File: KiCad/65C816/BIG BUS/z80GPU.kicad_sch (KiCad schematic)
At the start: 12 parts, among them J8 Bus Header, U12 74LS573, U13 74LS573, U14 74LS573, U15 74HC00, U16 CTC, U17 74HC02

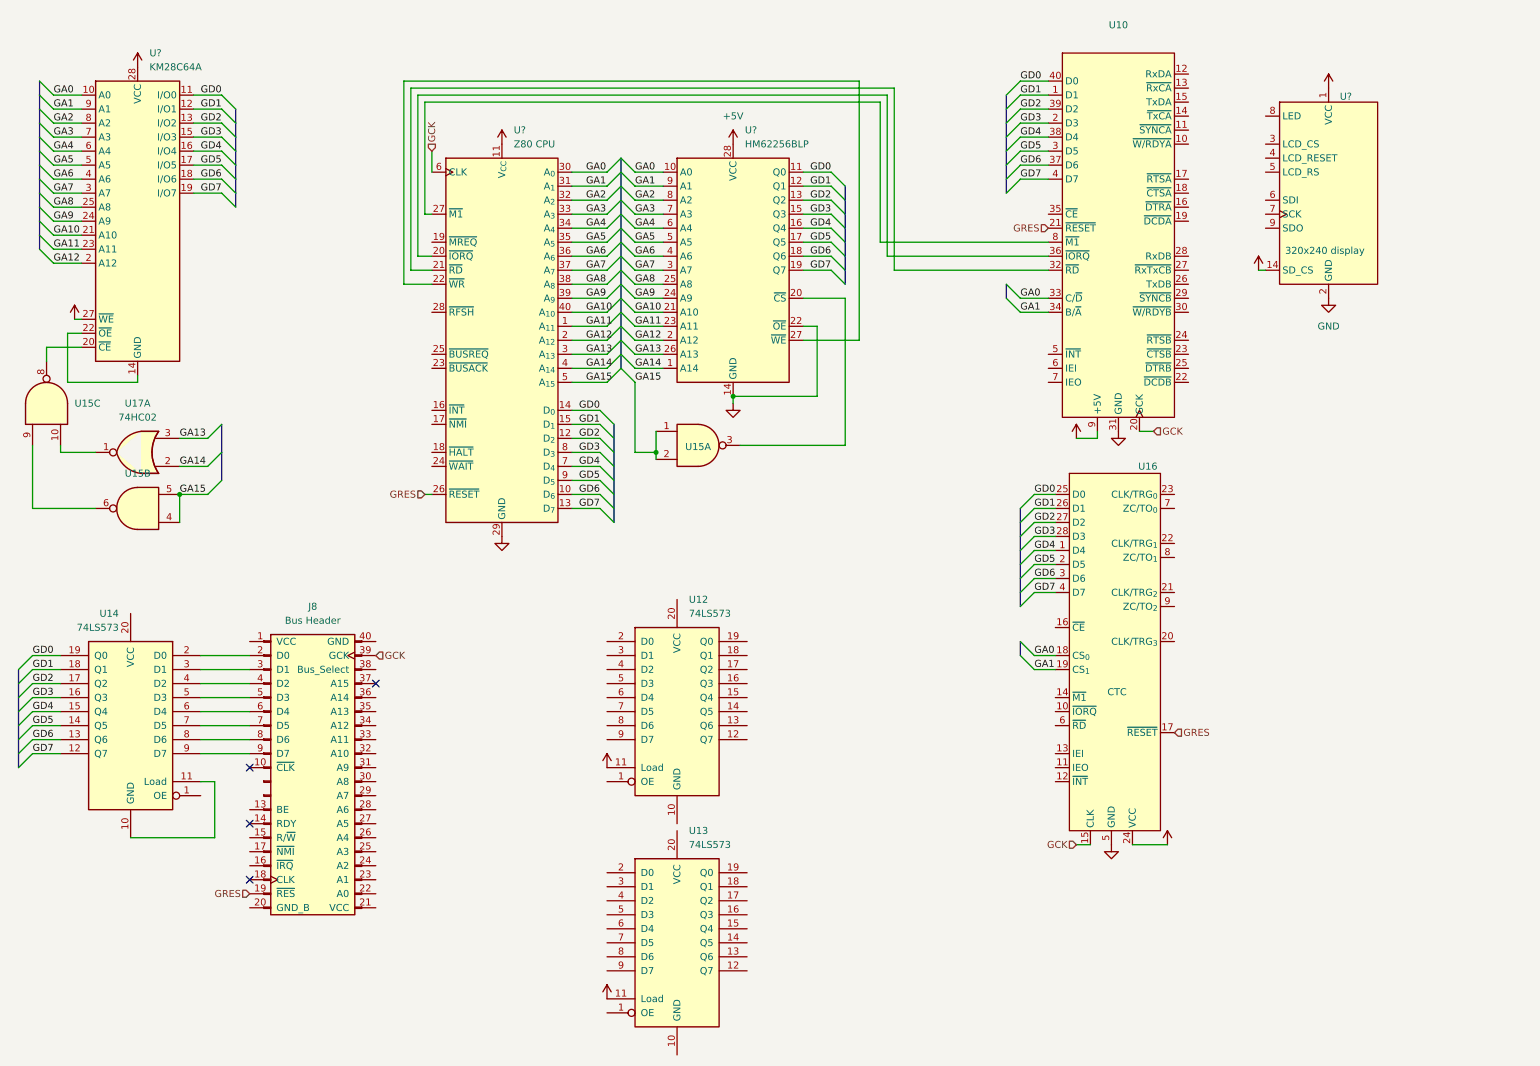
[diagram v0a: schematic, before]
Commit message: Preliminary PLD stuff, state machines are scary
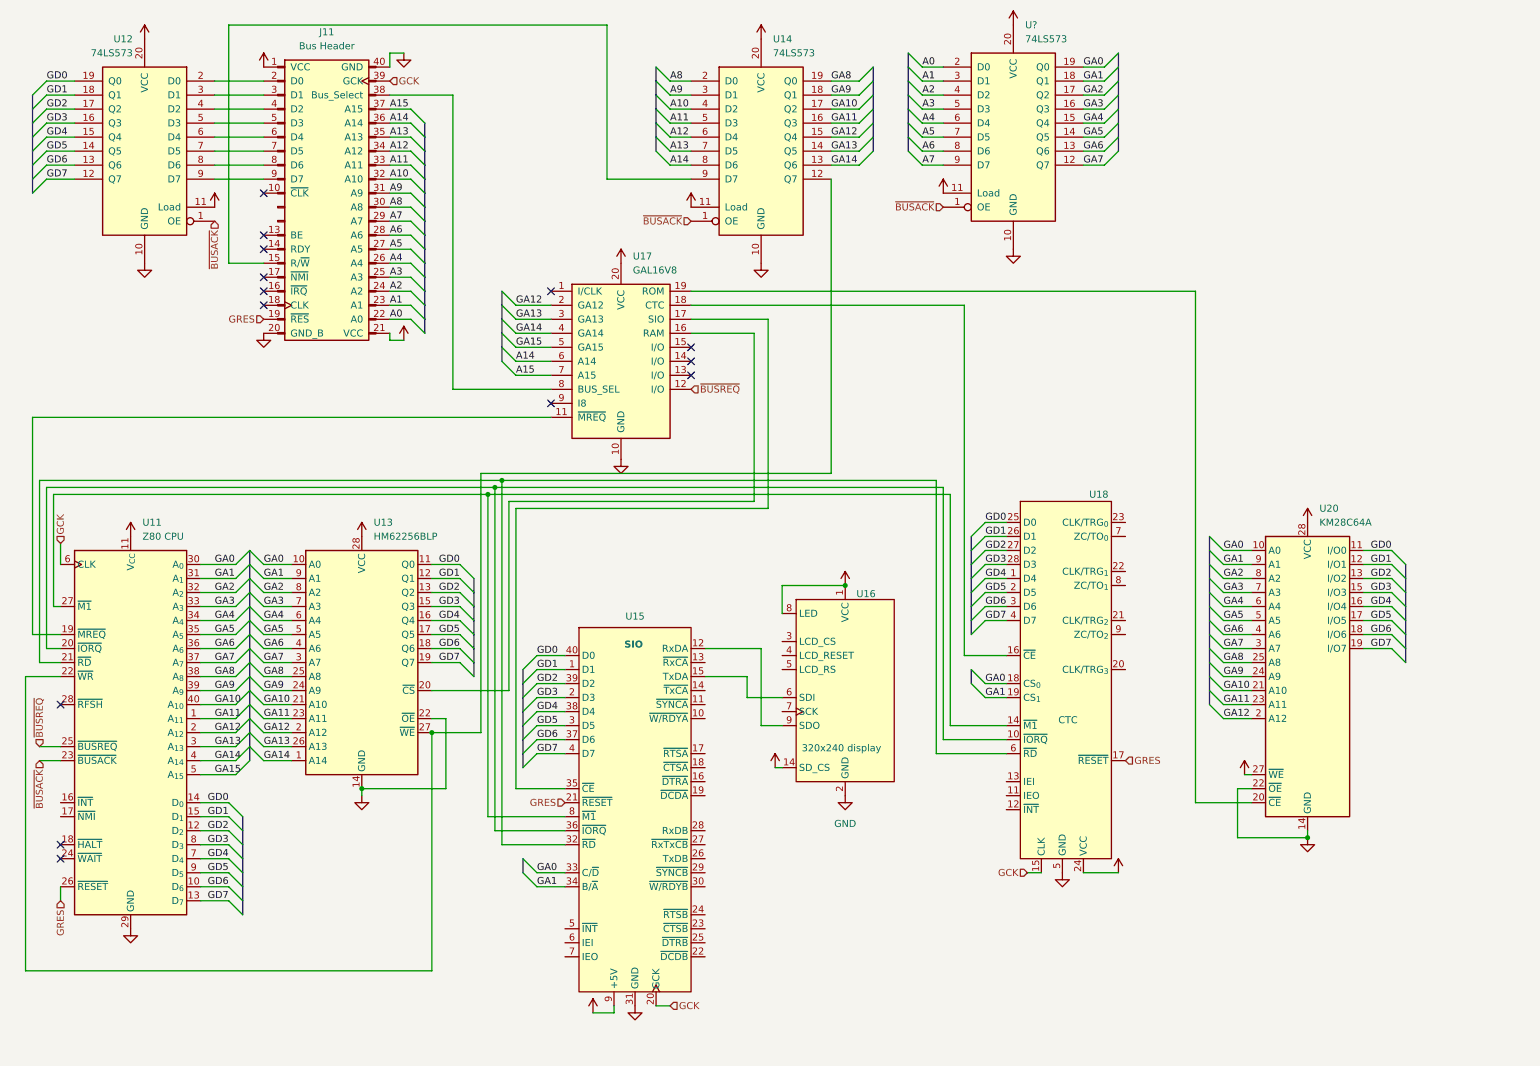
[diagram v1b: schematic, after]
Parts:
- removed U13: 74LS573, symbol 74xx:74LS573
- removed U15: 74HC00, symbol 74xx:74HC00
- removed U17: 74HC02, symbol 74xx:74HC02
- added U14: 74LS573, symbol 74xx:74LS573
- added U17: GAL16V8, Package_DIP:DIP-20_W7.62mm_Socket, symbol Board Connectors:GPU Bus Decode
- U15: renamed from U10; value ~ -> SIO
- gave numbers to parts that had none: 4
- renumbered J8 to J11, U14 to U12, U16 to U18, U12 to U?
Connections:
- net +5V: now also J11.1 (VCC), J11.21 (VCC), U12.11 (Load), U12.20 (VCC), U16.8 (LED), U?.20 (VCC), U14.11 (Load), U14.20 (VCC), U17.20 (VCC)
- net GA0: now also U?.19 (Q0)
- net GA1: now also U?.18 (Q1)
- net GA10: now also U14.17 (Q2)
- net GA11: now also U14.16 (Q3)
- net GA12: now also U14.15 (Q4), U17.2 (GA12)
- net GA13: now also U14.14 (Q5), U17.3 (GA13)
- net GA14: now also U14.13 (Q6), U17.4 (GA14)
- net GA15: now also U17.5 (GA15)
- net GA2: now also U?.17 (Q2)
- net GA3: now also U?.16 (Q3)
- net GA4: now also U?.15 (Q4)
- net GA5: now also U?.14 (Q5)
- net GA6: now also U?.13 (Q6)
- net GA7: now also U?.12 (Q7)
- net GA8: now also U14.19 (Q0)
- net GA9: now also U14.18 (Q1)
- net GND: now also J11.20 (GND_B), J11.40 (GND), U12.10 (GND), U20.14 (GND), U20.22 (~{OE}), U?.10 (GND), U14.10 (GND), U17.10 (GND)
- net at U20.20 (~{CE}): now also U17.19 (ROM)
- net at J11.15 (R/~{W}): now also U14.9 (D7)
- net A0: now reaches J11.22 (A0)
- net A0: now also U?.2 (D0)
- net A1: now reaches J11.23 (A1)
- net A1: now also U?.3 (D1)
- net A2: now reaches J11.24 (A2)
- net A2: now also U?.4 (D2)
- net A3: now reaches J11.25 (A3)
- net A3: now also U?.5 (D3)
- net A4: now reaches J11.26 (A4)
- net A4: now also U?.6 (D4)
- net A5: now reaches J11.27 (A5)
- net A5: now also U?.7 (D5)
- net A6: now reaches J11.28 (A6)
- net A6: now also U?.8 (D6)
- net A7: now reaches J11.29 (A7)
- net A7: now also U?.9 (D7)
- net A8: now reaches J11.30 (A8)
- net A8: now also U14.2 (D0)
- net A9: now reaches J11.31 (A9)
- net A9: now also U14.3 (D1)
- net A10: now reaches J11.32 (A10)
- net A10: now also U14.4 (D2)
- net A11: now reaches J11.33 (A11)
- net A11: now also U14.5 (D3)
- net A12: now reaches J11.34 (A12)
- net A12: now also U14.6 (D4)
- net A13: now reaches J11.35 (A13)
- net A13: now also U14.7 (D5)
- net A14: now reaches J11.36 (A14)
- net A14: now also U14.8 (D6), U17.6 (A14)
- net A15: now reaches J11.37 (A15)
- net A15: now also U17.7 (A15)
- net at J11.38 (Bus_Select): now also U17.8 (BUS_SEL)
- net at U11.19 (~{MREQ}): now also U17.11 (~{MREQ})
- net at U11.20 (~{IORQ}), U15.36 (~{IORQ}): now also U18.10 (~{IORQ})
- net at U11.21 (~{RD}), U15.32 (~{RD}): now also U18.6 (~{RD})
- net at U11.22 (~{WR}), U13.27 (~{WE}): now also U14.12 (Q7)
- net ~{BUSACK}: now reaches U11.23 (~{BUSACK})
- net ~{BUSACK}: now also U12.1 (OE), U?.1 (OE), U14.1 (OE)
- net ~{BUSREQ}: now reaches U11.25 (~{BUSREQ})
- net ~{BUSREQ}: now also U17.12 (I/O)
- net at U11.27 (~{M1}), U15.8 (~{M1}): now also U18.14 (~{M1})
- net at U18.16 (~{CE}): now also U17.18 (CTC)
- net at U13.20 (~{CS}): now also U17.16 (RAM)
- net at U15.12 (RxDA): now also U16.9 (SDO)
- net at U15.15 (TxDA): now also U16.6 (SDI)
- net at U15.35 (~{CE}): now also U17.17 (SIO)
- no-connect marks 4 -> 14
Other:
- moved on the sheet: J11, U11, U12, U13, U15, U16, U18, U20, U?

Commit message: lots of stiff
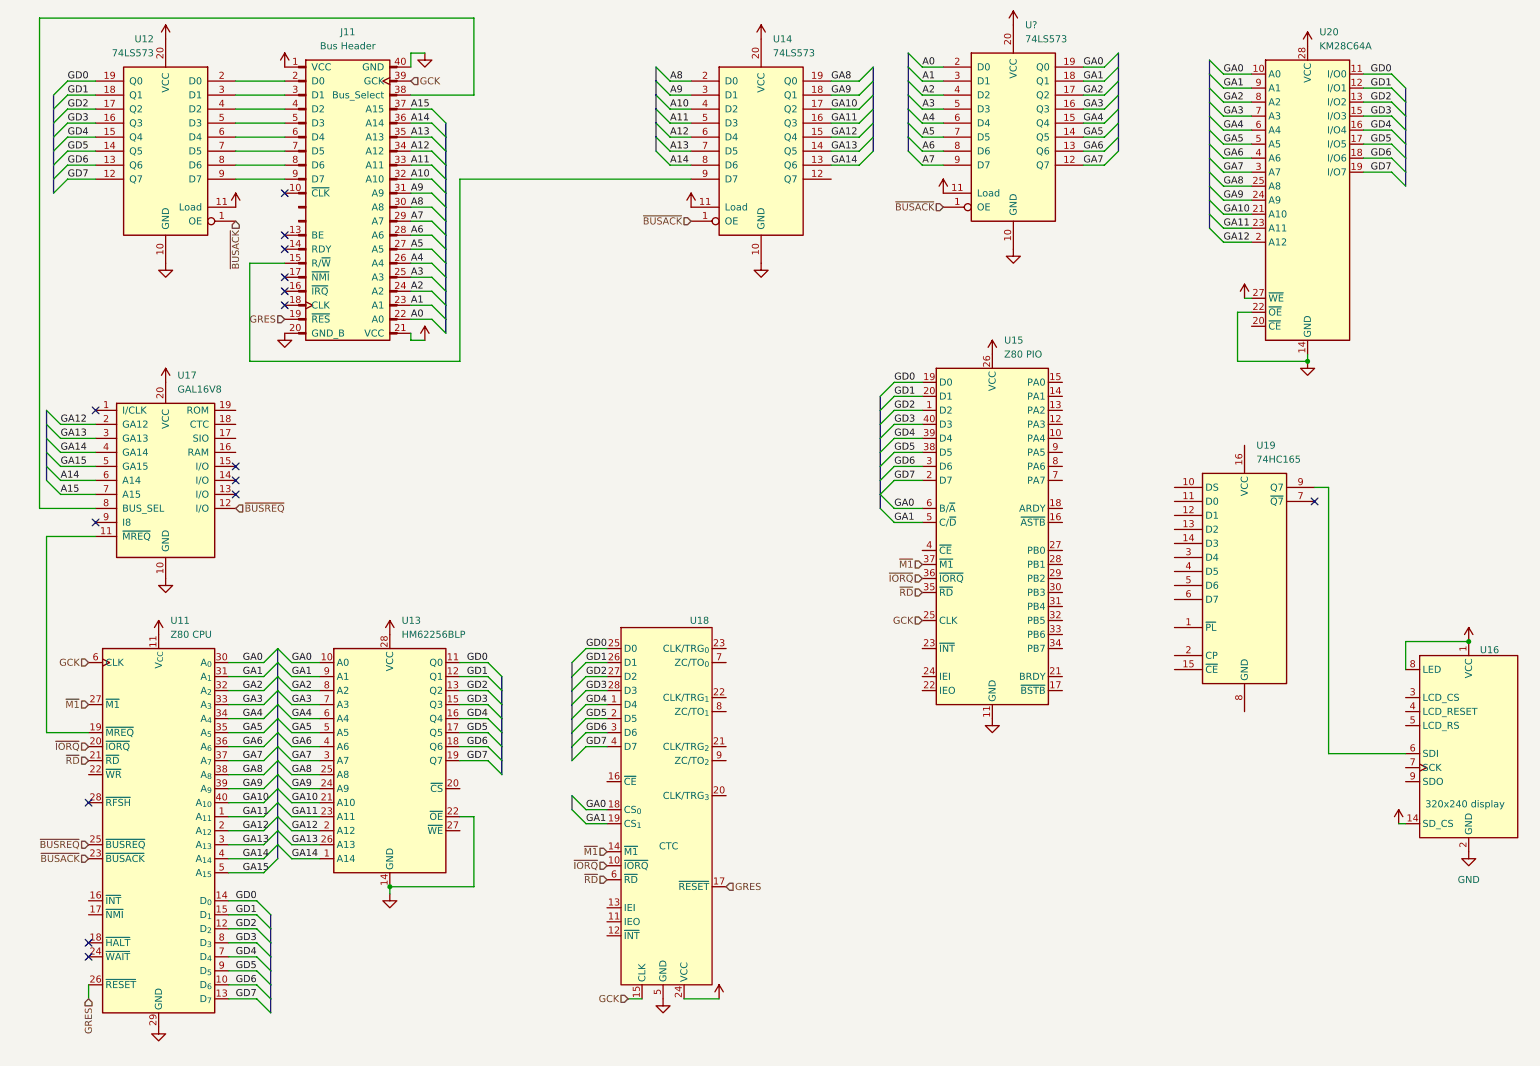
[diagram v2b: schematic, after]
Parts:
- removed U15: SIO, Package_DIP:DIP-40_W15.24mm_Socket, symbol Board Connectors:Z80_SIO
- added U15: Z80 PIO, Package_DIP:DIP-40_W15.24mm, symbol Interface:Z8420
- added U19: 74HC165, symbol 74xx:74HC165
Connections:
- net +5V: now also U15.26 (VCC)
- net GA0: now also U15.6 (B/~{A})
- net GA1: now also U15.5 (C/~{D})
- net GCK: now also U15.25 (CLK)
- net GD0: now also U15.19 (D0)
- net GD1: now also U15.20 (D1)
- net GD2: now also U15.1 (D2)
- net GD3: now also U15.40 (D3)
- net GD4: now also U15.39 (D4)
- net GD5: now also U15.38 (D5)
- net GD6: now also U15.3 (D6)
- net GD7: now also U15.2 (D7)
- net GND: now also U15.11 (GND)
- net at U20.20 (~{CE}): no longer U17.19 (ROM)
- net ~{IORQ}: now reaches U11.20 (~{IORQ}), U18.10 (~{IORQ})
- net ~{IORQ}: now also U15.36 (~{IORQ})
- net ~{RD}: now reaches U11.21 (~{RD}), U18.6 (~{RD})
- net ~{RD}: now also U15.35 (~{RD})
- net ~{M1}: now reaches U11.27 (~{M1}), U18.14 (~{M1})
- net ~{M1}: now also U15.37 (~{M1})
- net at U18.16 (~{CE}): no longer U17.18 (CTC)
- net at U13.20 (~{CS}): no longer U17.16 (RAM)
- net at U16.6 (SDI): now also U19.9 (Q7)
- now unconnected: U11.22 (~{WR}), U13.27 (~{WE}), U14.12 (Q7)
- no-connect marks 14 -> 15
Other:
- moved on the sheet: J11, U11, U12, U13, U17, U18, U20
